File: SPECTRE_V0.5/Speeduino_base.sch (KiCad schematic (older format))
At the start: 214 parts, among them J1 Conn_01x04_Male, J2 Conn_02x04_Odd_Even, J3 Conn_01x06_Male, Q1 2N7002, Q10 BSP78, Q11 BSP78, Q12 BSP78, Q13 BSP78, Q14 BSP78, Q15 BSP78, Q16 SMD-MOSFET-N-CH-55V-2.1A-AO34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, Q17 AO3401A, Q18 BSP78, Q19 SMD-MOSFET-N-CH-55V-2.1A-AO34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, Q2 CJ2302, Q20 AO3401A, Q21 SMD-MOSFET-N-CH-55V-2.1A-AO34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, Q22 SMD-MOSFET-N-CH-55V-2.1A-AO34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, Q23 AO3401A, Q24 AO3401A, Q25 BSP78, Q26 BSP78, Q3 CJ2302, Q4 CJ2302, Q5 BSP78, Q6 BSP78, Q7 CJ2302, Q8 CJ2302, Q9 CJ2302, U1 MAX9926UAEE+, U2 molex_48pin, U3 LM78M05_TO220, U4 MAX3232

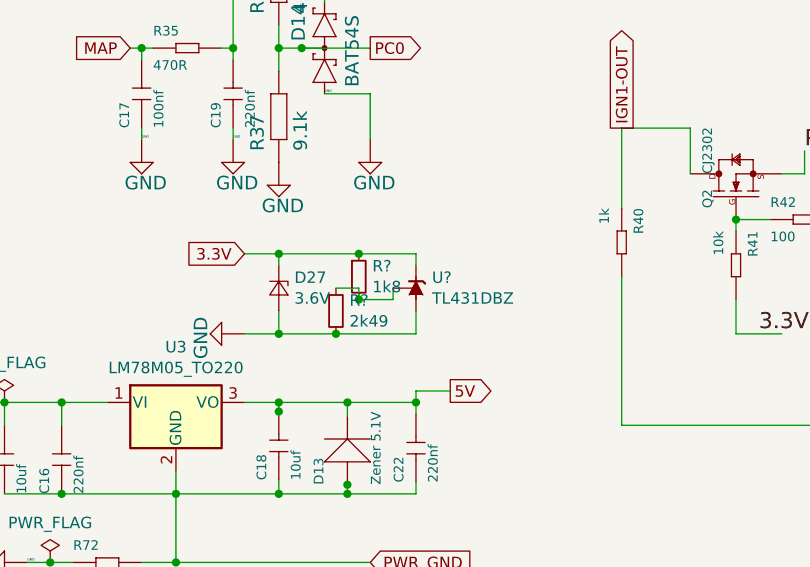
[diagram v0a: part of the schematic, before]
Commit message: Update Speeduino_base.sch
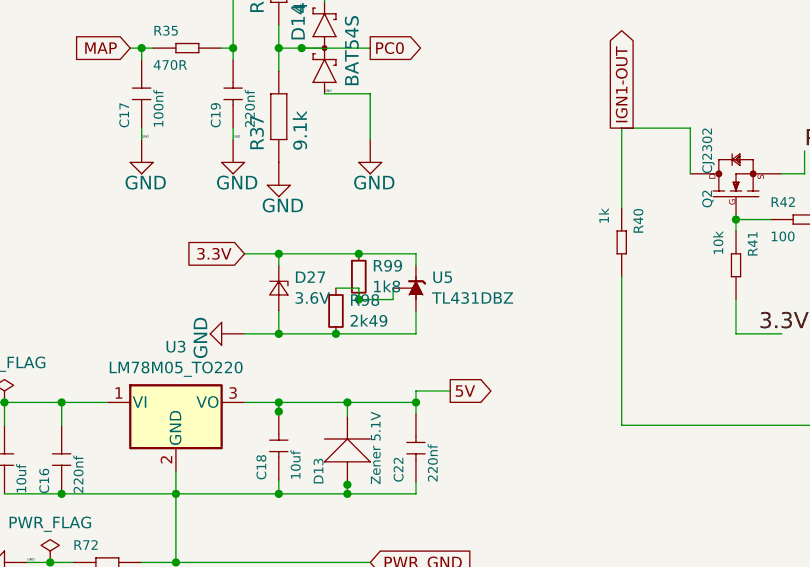
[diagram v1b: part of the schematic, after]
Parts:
- gave numbers to parts that had none: 3
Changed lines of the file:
@@
 NoConn ~ 10200 4500
 $Comp
-L Reference_Voltage:TL431DBZ U?
+L Reference_Voltage:TL431DBZ U5
 U 1 1 5EC38137
 P 3750 10300
-F 0 "U?" V 3796 10230 50  0000 R CNN
+F 0 "U5" V 3796 10230 50  0000 R CNN
 F 1 "TL431DBZ" V 3705 10230 50  0000 R CNN
 F 2 "Package_TO_SOT_SMD:SOT-23" H 3750 10150 50  0001 C CIN
@@
 Connection ~ 3150 10500
 $Comp
-L Device:R_Small R?
+L Device:R_Small R99
 U 1 1 5ECE80FF
 P 3500 10250
-F 0 "R?" H 3559 10296 50  0000 L CNN
+F 0 "R99" H 3559 10296 50  0000 L CNN
 F 1 "1k8" H 3559 10205 50  0000 L CNN
 F 2 "Resistor_SMD:R_0603_1608Metric_Pad1.05x0.95mm_HandSolder" H 3500 10250 50  0001 C CNN
@@
 	3500 10150 3750 10150
 $Comp
-L Device:R_Small R?
+L Device:R_Small R98
 U 1 1 5ECEB0D8
 P 3400 10400
-F 0 "R?" H 3459 10446 50  0000 L CNN
+F 0 "R98" H 3459 10446 50  0000 L CNN
 F 1 "2k49" H 3459 10355 50  0000 L CNN
 F 2 "Resistor_SMD:R_0603_1608Metric_Pad1.05x0.95mm_HandSolder" H 3400 10400 50  0001 C CNN
